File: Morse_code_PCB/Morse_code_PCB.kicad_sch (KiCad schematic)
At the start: 60 parts, among them J1 USB_C_Receptacle_USB2.0, J2 INPUT, J3 OUTPUT, J4 Conn_01x02_Female, Q1 AO3400A, Q2 AO3401A, Q3 AO3400A, Q4 AO3401A, SW1 RotaryEncoder_Switch, U1 STM32F030F4Px, U2 OLED_12864, U3 MCP73831-2-OT, U4 CH340E, U5 LP5907MFX-3.3, U6 24AA02-OT

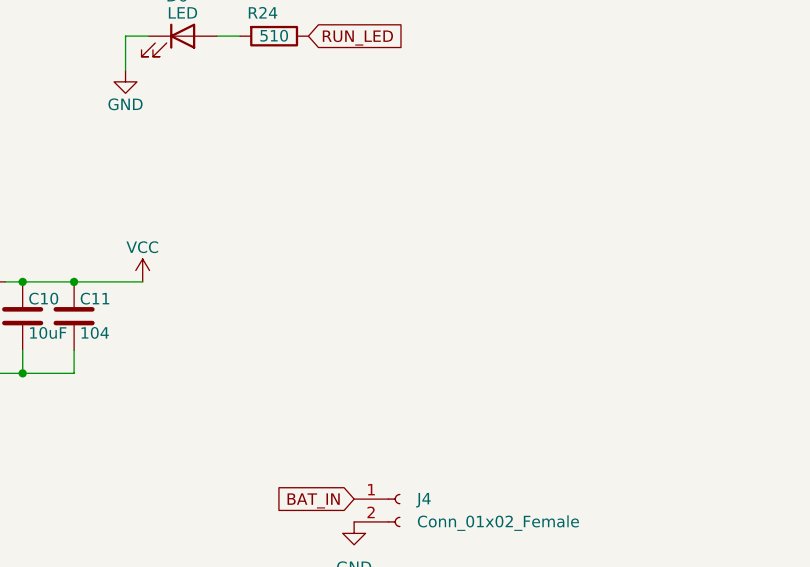
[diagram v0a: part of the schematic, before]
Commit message: PCB画完 Signed-off-by: kevin <kevin@lmve.net>
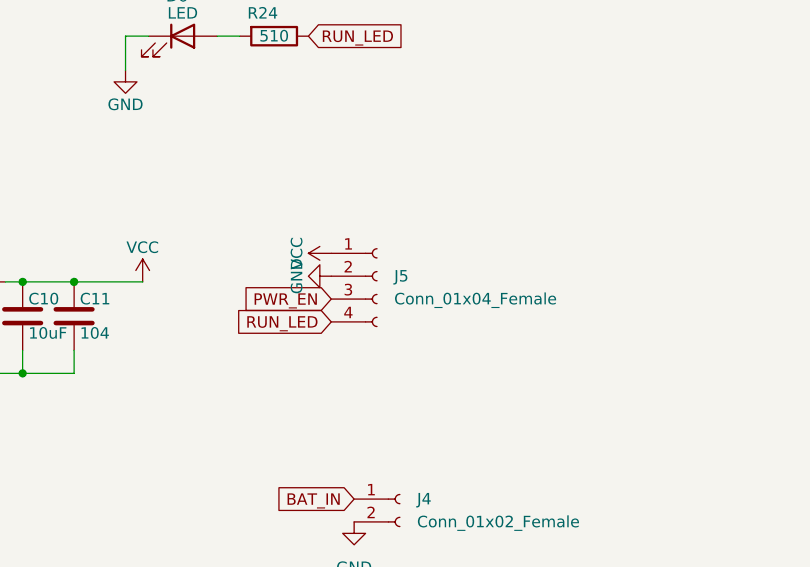
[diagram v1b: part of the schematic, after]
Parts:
- added J5: Conn_01x04_Female, MY:SIP-4, symbol Connector:Conn_01x04_Female
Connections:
- net GND: now also J5.2 (Pin_2)
- net PWR_EN: now also J5.3 (Pin_3)
- net RUN_LED: now also J5.4 (Pin_4)
- net VCC: now also J5.1 (Pin_1)
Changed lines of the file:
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@@
+    )
+  )
+  (global_label "RUN_LED" (shape input) (at 142.875 115.57 180) (fields_autoplaced)
+    (effects (font (size 1.27 1.27)) (justify right))
+    (property "插入图纸页参考" "${INTERSHEET_REFS}" (id 0) (at 132.1162 115.6494 0)
+      (effects (font (size 1.27 1.27)) (justify right) hide)
     )
   )
@@
     (property "插入图纸页参考" "${INTERSHEET_REFS}" (id 0) (at 64.6431 181.5306 0)
       (effects (font (size 1.27 1.27)) (justify left) hide)
+    )
+  )
+  (global_label "PWR_EN" (shape input) (at 142.875 113.03 180) (fields_autoplaced)
+    (effects (font (size 1.27 1.27)) (justify right))
+    (property "Intersheet References" "${INTERSHEET_REFS}" (id 0) (at 133.0233 113.1094 0)
+      (effects (font (size 1.27 1.27)) (justify right) hide)
     )
   )
@@
     (pin "8")
     (pin "9")
+  )
+  (symbol (lib_id "power:VCC") (at 142.875 107.95 90) (unit 1)
+    (in_bom yes) (on_board yes)
+    (property "Reference" "#PWR0121" (id 0) (at 146.685 107.95 0)
+      (effects (font (size 1.27 1.27)) hide)
+    )
+    (property "Value" "VCC" (id 1) (at 139.065 107.95 0))
+    (property "Footprint" "" (id 2) (at 142.875 107.95 0)
+      (effects (font (size 1.27 1.27)) hide)
+    )
+    (property "Datasheet" "" (id 3) (at 142.875 107.95 0)
+      (effects (font (size 1.27 1.27)) hide)
+    )
+    (pin "1")
   )
   (symbol (lib_id "Device:R") (at 48.895 36.83 270) (unit 1)
@@
     (pin "2")
   )
+  (symbol (lib_id "power:GND") (at 142.875 110.49 270) (unit 1)
+    (in_bom yes) (on_board yes)
+    (property "Reference" "#PWR0120" (id 0) (at 136.525 110.49 0)
+      (effects (font (size 1.27 1.27)) hide)
+    )
+    (property "Value" "GND" (id 1) (at 139.065 110.49 0))
+    (property "Footprint" "" (id 2) (at 142.875 110.49 0)
+      (effects (font (size 1.27 1.27)) hide)
+    )
+    (property "Datasheet" "" (id 3) (at 142.875 110.49 0)
+      (effects (font (size 1.27 1.27)) hide)
+    )
+    (pin "1")
+  )
   (symbol (lib_id "Transistor_FET:AO3401A") (at 246.38 71.755 180) (unit 1)
     (in_bom yes) (on_board yes)
@@
     (pin "1")
     (pin "2")
+  )
+  (symbol (lib_id "Connector:Conn_01x04_Female") (at 147.955 110.49 0) (unit 1)
+    (in_bom yes) (on_board yes) (fields_autoplaced)
+    (property "Reference" "J5" (id 0) (at 149.86 110.4899 0)
+      (effects (font (size 1.27 1.27)) (justify left))
+    )
+    (property "Value" "Conn_01x04_Female" (id 1) (at 149.86 113.0299 0)
+      (effects (font (size 1.27 1.27)) (justify left))
+    )
+    (property "Footprint" "MY:SIP-4" (id 2) (at 147.955 110.49 0)
+      (effects (font (size 1.27 1.27)) hide)
+    )
+    (property "Datasheet" "~" (id 3) (at 147.955 110.49 0)
+      (effects (font (size 1.27 1.27)) hide)
+    )
+    (pin "1")
+    (pin "2")
+    (pin "3")
+    (pin "4")
   )
   (symbol (lib_id "Device:R") (at 234.95 100.33 180) (unit 1)
@@
       (reference "#PWR0119") (unit 1) (value "GND") (footprint "")
     )
+    (path "/8db05113-bb5d-40cb-916f-5b0147562482"
+      (reference "#PWR0120") (unit 1) (value "GND") (footprint "")
+    )
+    (path "/4bc53345-25fe-427a-a648-514d97b80f54"
+      (reference "#PWR0121") (unit 1) (value "VCC") (footprint "")
+    )
     (path "/972eb069-8d6d-41f6-83d3-1d7e45627208"
       (reference "BZ1") (unit 1) (value "Buzzer") (footprint "Buzzer_Beeper:Buzzer_TDK_PS1240P02BT_D12.2mm_H6.5mm")
@@
       (reference "J4") (unit 1) (value "Conn_01x02_Female") (footprint "MY:SIP-2")
     )
+    (path "/9f9d9ec1-f12a-47cb-a033-e6a9e0eb276a"
+      (reference "J5") (unit 1) (value "Conn_01x04_Female") (footprint "MY:SIP-4")
+    )
     (path "/a6e73968-bfeb-49ba-b5d0-6a71117f7ee3"

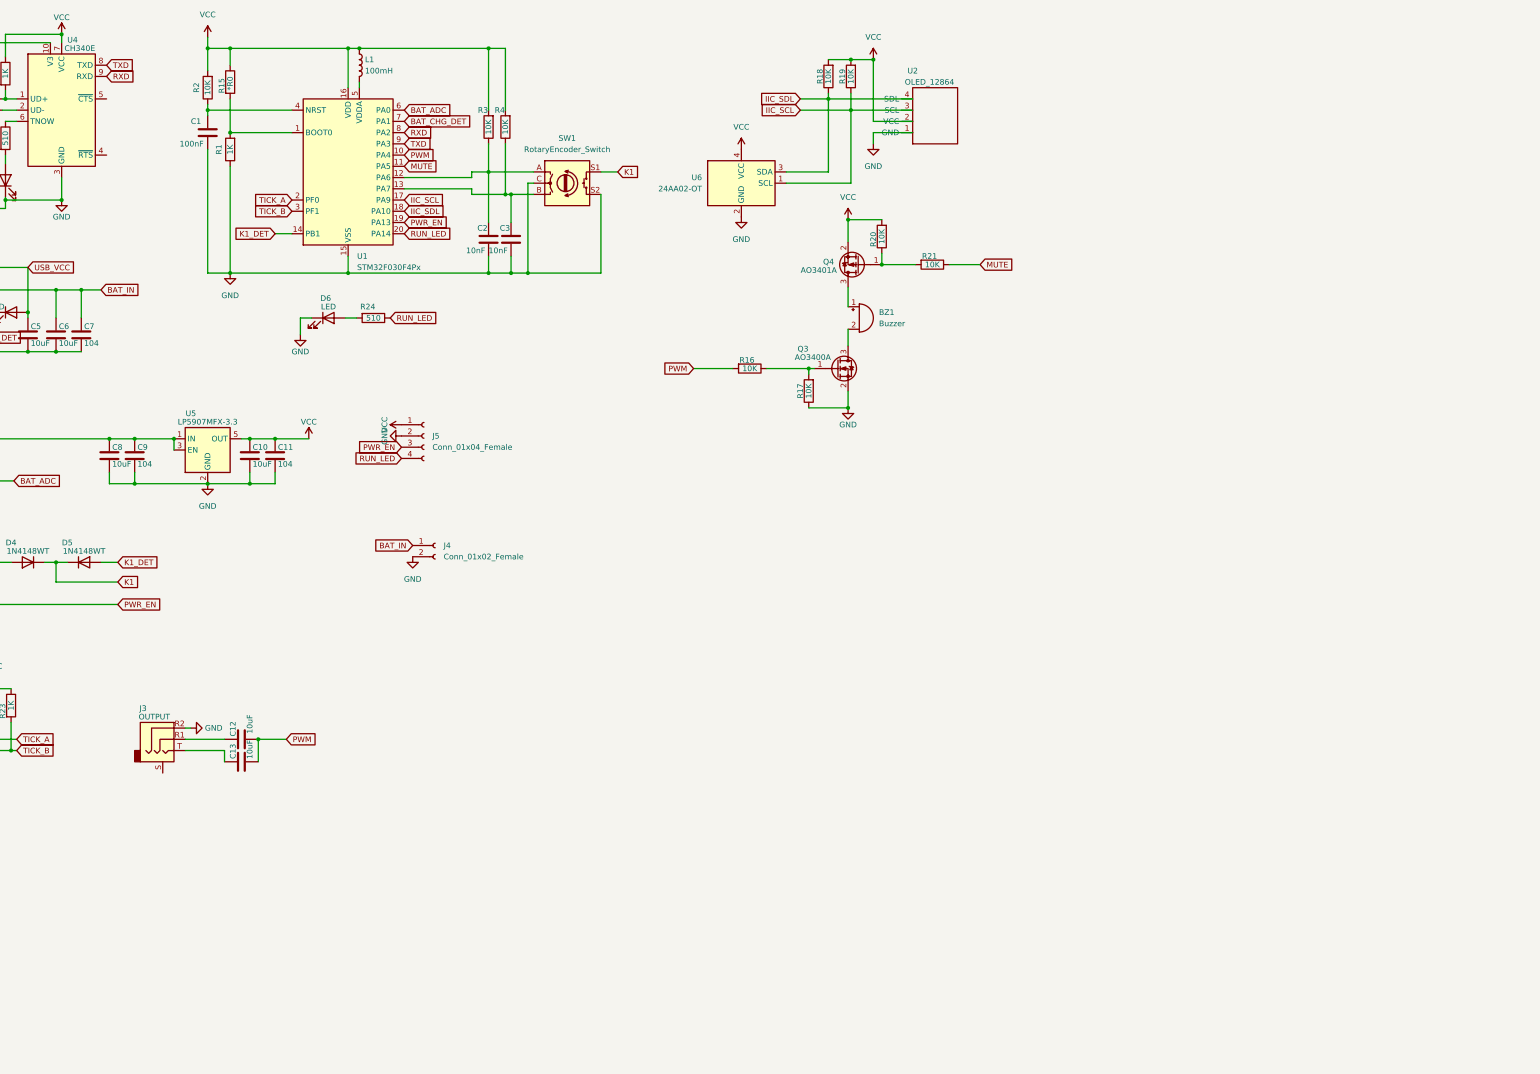
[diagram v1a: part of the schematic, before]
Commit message: PCB updata Signed-off-by: kevin <kevin@lmve.net>
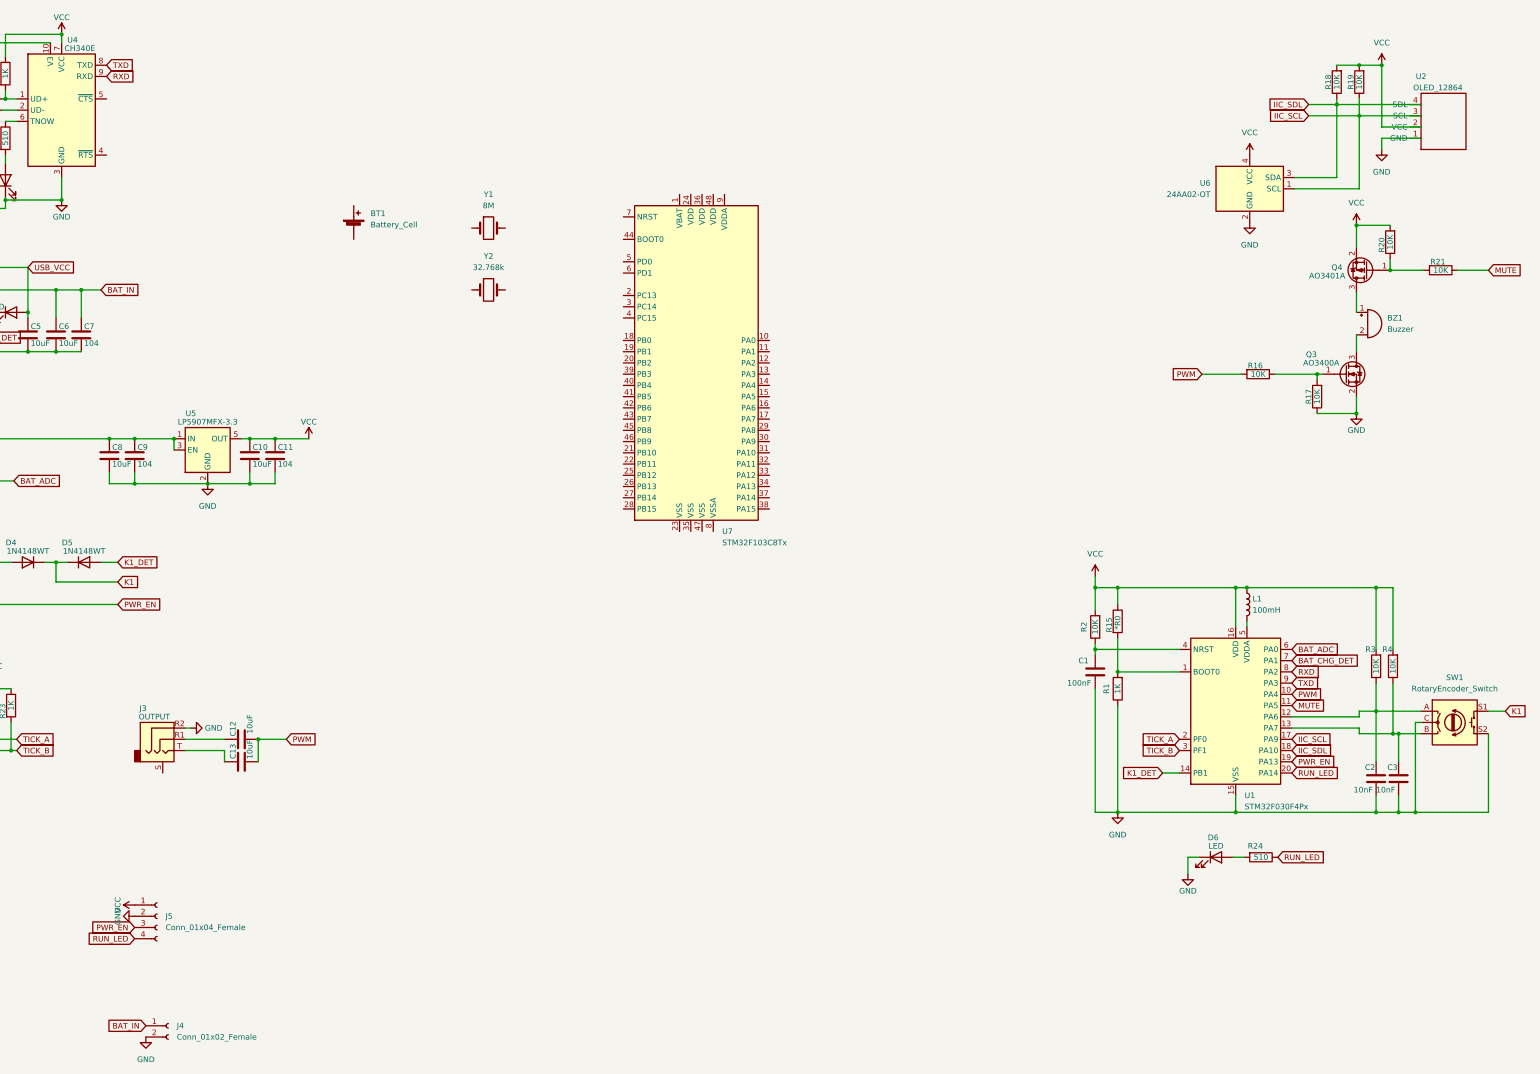
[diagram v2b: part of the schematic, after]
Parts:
- added BT1: Battery_Cell, MY:BAT_BC501SM, symbol Device:Battery_Cell
- added U7: STM32F103C8Tx, Package_QFP:LQFP-48_7x7mm_P0.5mm, symbol MCU_ST_STM32F1:STM32F103C8Tx
- added Y1: 8M, Crystal:Crystal_SMD_5032-2Pin_5.0x3.2mm, symbol Device:Crystal
- added Y2: 32.768k, Crystal:Crystal_SMD_3215-2Pin_3.2x1.5mm, symbol Device:Crystal
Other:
- moved on the sheet: BZ1, C1, C2, C3, D6, J4, J5, L1, Q3, Q4, R1, R15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
